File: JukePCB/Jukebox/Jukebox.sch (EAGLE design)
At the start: 31 parts, among them CN1 1X4-BIG

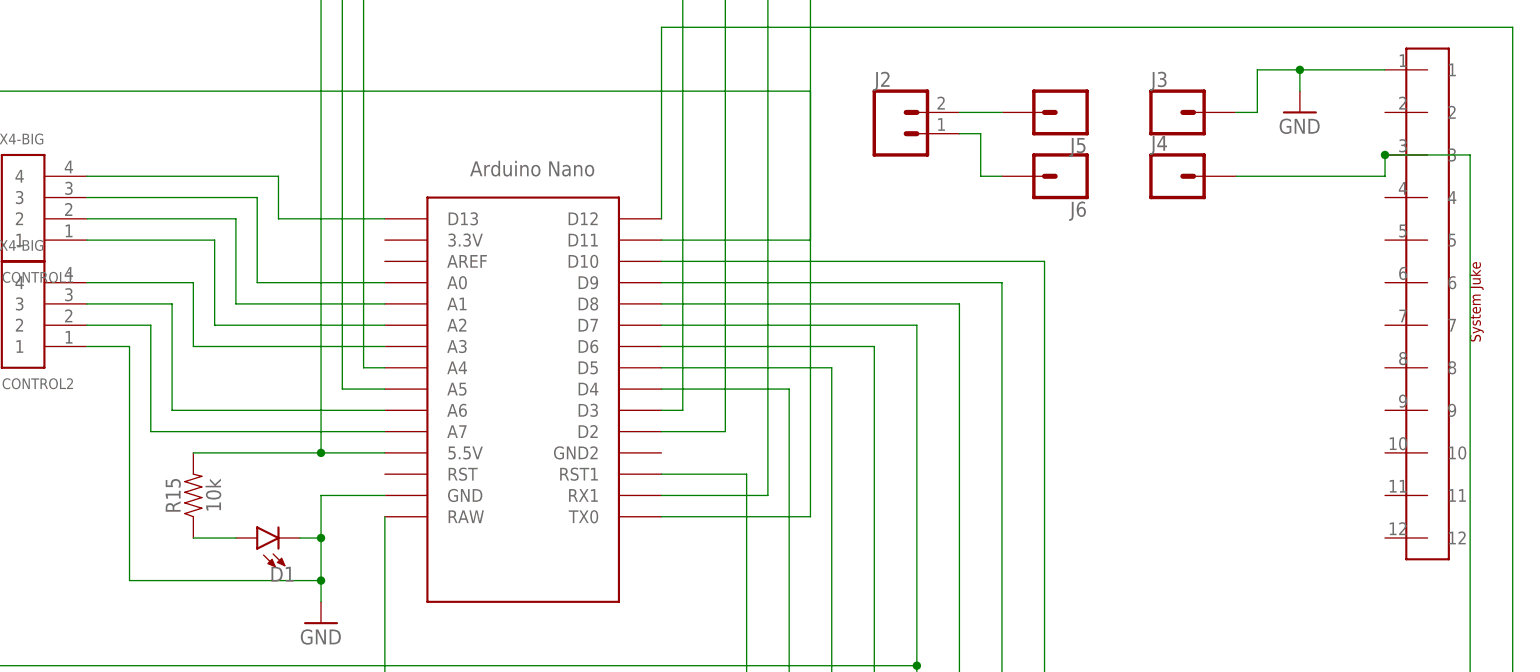
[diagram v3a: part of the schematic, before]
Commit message: board proto 1
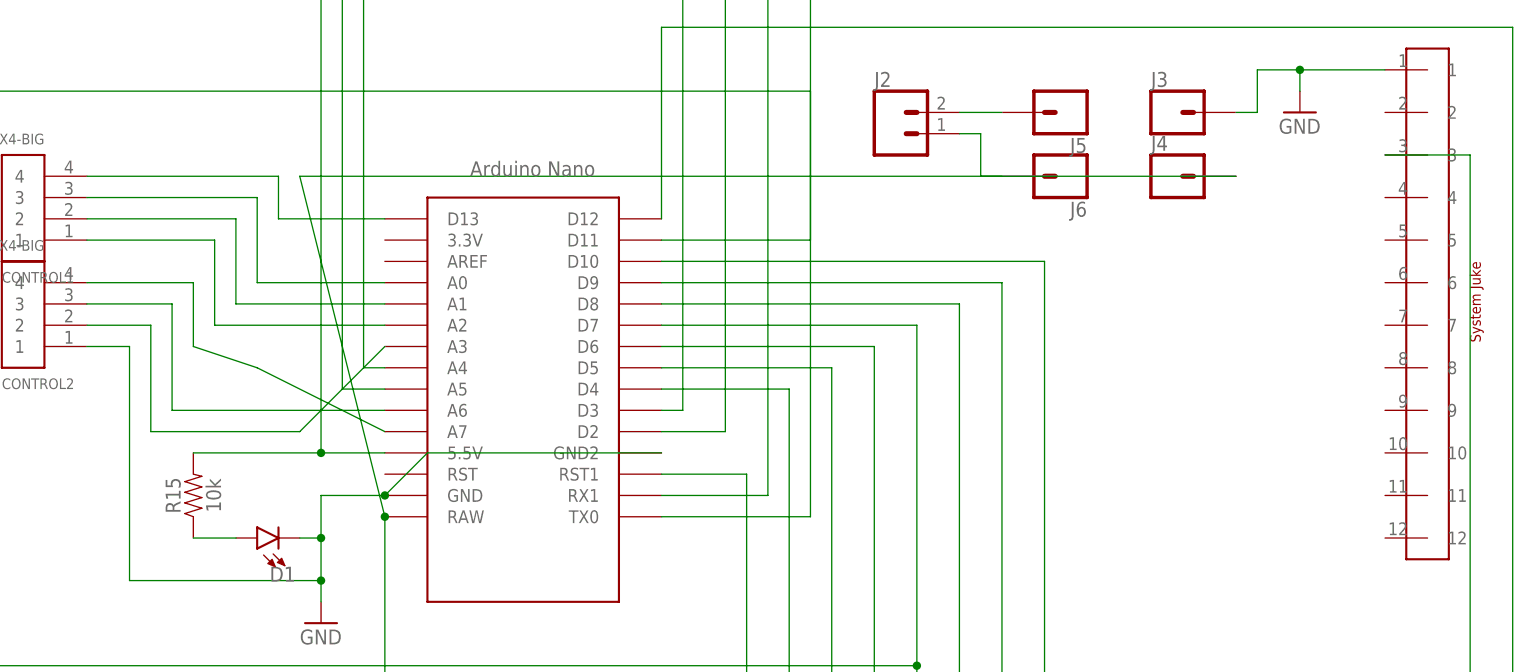
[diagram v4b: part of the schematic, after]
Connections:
- net GND: now also U$1.GND2
- net N$31: now also U$1.A7; no longer U$1.A3
- net N$32: now also J4.1
- net N$36: now also U$1.A3; no longer U$1.A7
- net N$8: no longer J4.1
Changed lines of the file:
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@@
 <wire x1="86.36" y1="-55.88" x2="86.36" y2="2.54" width="0.1524" layer="91"/>
 <pinref part="U$1" gate="G$1" pin="D10"/>
-<wire x1="86.36" y1="2.54" x2="40.64" y2="2.54" width="0.1524" layer="91"/>
+<wire x1="40.64" y1="2.54" x2="86.36" y2="2.54" width="0.1524" layer="91"/>
 </segment>
 </net>
@@
 <pinref part="U$14" gate="G$1" pin="3"/>
 <wire x1="137.16" y1="-127" x2="68.58" y2="-127" width="0.1524" layer="91"/>
-<pinref part="J4" gate="G$1" pin="1"/>
-<wire x1="109.22" y1="12.7" x2="127" y2="12.7" width="0.1524" layer="91"/>
-<wire x1="127" y1="12.7" x2="127" y2="15.24" width="0.1524" layer="91"/>
-<junction x="127" y="15.24"/>
 </segment>
 </net>
@@
 <wire x1="45.72" y1="-93.98" x2="7.62" y2="-93.98" width="0.1524" layer="91"/>
 <wire x1="7.62" y1="-93.98" x2="7.62" y2="-27.94" width="0.1524" layer="91"/>
+<pinref part="J4" gate="G$1" pin="1"/>
+<wire x1="109.22" y1="12.7" x2="-2.54" y2="12.7" width="0.1524" layer="91"/>
+<wire x1="-2.54" y1="12.7" x2="7.62" y2="-27.94" width="0.1524" layer="91"/>
+<junction x="7.62" y="-27.94"/>
 </segment>
 </net>
@@
 <pinref part="CONTROL2" gate="G$1" pin="1"/>
 <wire x1="-22.86" y1="-7.62" x2="-27.94" y2="-7.62" width="0.1524" layer="91"/>
+<pinref part="U$1" gate="G$1" pin="GND2"/>
+<wire x1="40.64" y1="-20.32" x2="12.7" y2="-20.32" width="0.1524" layer="91"/>
+<wire x1="12.7" y1="-20.32" x2="7.62" y2="-25.4" width="0.1524" layer="91"/>
+<junction x="7.62" y="-25.4"/>
 </segment>
 </net>
@@
 <wire x1="-27.94" y1="0" x2="-15.24" y2="0" width="0.1524" layer="91"/>
 <wire x1="-15.24" y1="0" x2="-15.24" y2="-7.62" width="0.1524" layer="91"/>
-<pinref part="U$1" gate="G$1" pin="A3"/>
-<wire x1="-15.24" y1="-7.62" x2="7.62" y2="-7.62" width="0.1524" layer="91"/>
+<pinref part="U$1" gate="G$1" pin="A7"/>
+<wire x1="-15.24" y1="-7.62" x2="-7.62" y2="-10.16" width="0.1524" layer="91"/>
+<wire x1="-7.62" y1="-10.16" x2="7.62" y2="-17.78" width="0.1524" layer="91"/>
 </segment>
 </net>
@@
 <wire x1="-27.94" y1="-5.08" x2="-20.32" y2="-5.08" width="0.1524" layer="91"/>
 <wire x1="-20.32" y1="-5.08" x2="-20.32" y2="-17.78" width="0.1524" layer="91"/>
-<pinref part="U$1" gate="G$1" pin="A7"/>
-<wire x1="-20.32" y1="-17.78" x2="7.62" y2="-17.78" width="0.1524" layer="91"/>
-</segment>
-</net>
+<pinref part="U$1" gate="G$1" pin="A3"/>
+<wire x1="-20.32" y1="-17.78" x2="-2.54" y2="-17.78" width="0.1524" layer="91"/>
+<wire x1="-2.54" y1="-17.78" x2="7.62" y2="-7.62" width="0.1524" layer="91"/>
+</segment>
+</net>

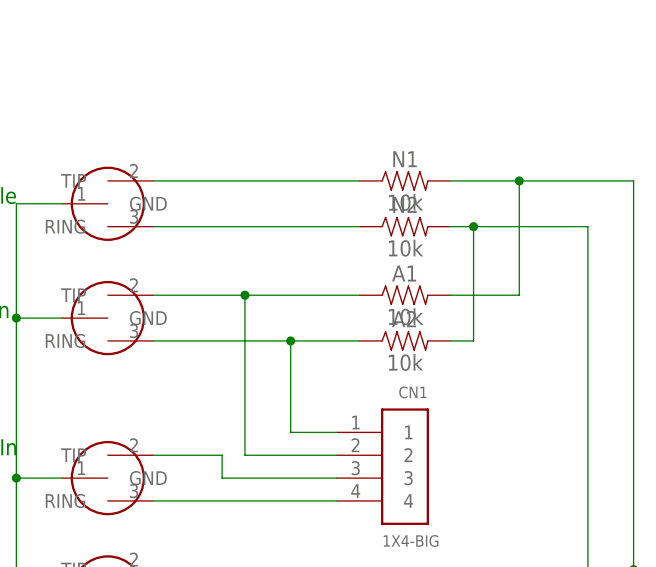
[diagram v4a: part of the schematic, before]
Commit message: almost final routes
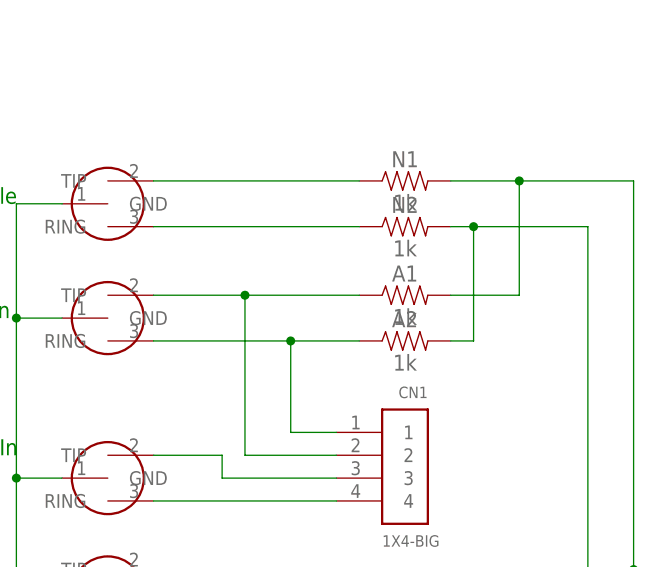
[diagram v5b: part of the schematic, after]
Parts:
- A1, A2, N1, N2: value 10k -> 1k
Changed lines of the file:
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@@
 <part name="TOAMP" library="Jukebox" deviceset="JUKEHEADPHONE" device=""/>
 <part name="AUXOUT" library="Jukebox" deviceset="JUKEHEADPHONE" device=""/>
-<part name="N1" library="SparkFun-Resistors" deviceset="10KOHM" device="-HORIZ-1/4W-1%" value="10k"/>
-<part name="N2" library="SparkFun-Resistors" deviceset="10KOHM" device="-HORIZ-1/4W-1%" value="10k"/>
-<part name="A1" library="SparkFun-Resistors" deviceset="10KOHM" device="-HORIZ-1/4W-1%" value="10k"/>
-<part name="A2" library="SparkFun-Resistors" deviceset="10KOHM" device="-HORIZ-1/4W-1%" value="10k"/>
+<part name="N1" library="SparkFun-Resistors" deviceset="10KOHM" device="-HORIZ-1/4W-1%" value="1k"/>
+<part name="N2" library="SparkFun-Resistors" deviceset="10KOHM" device="-HORIZ-1/4W-1%" value="1k"/>
+<part name="A1" library="SparkFun-Resistors" deviceset="10KOHM" device="-HORIZ-1/4W-1%" value="1k"/>
+<part name="A2" library="SparkFun-Resistors" deviceset="10KOHM" device="-HORIZ-1/4W-1%" value="1k"/>
 <part name="TOLIGHT" library="Jukebox" deviceset="JUKEHEADPHONE" device=""/>
 <part name="R15" library="SparkFun-Resistors" deviceset="10KOHM" device="-HORIZ-1/4W-1%" value="10k"/>

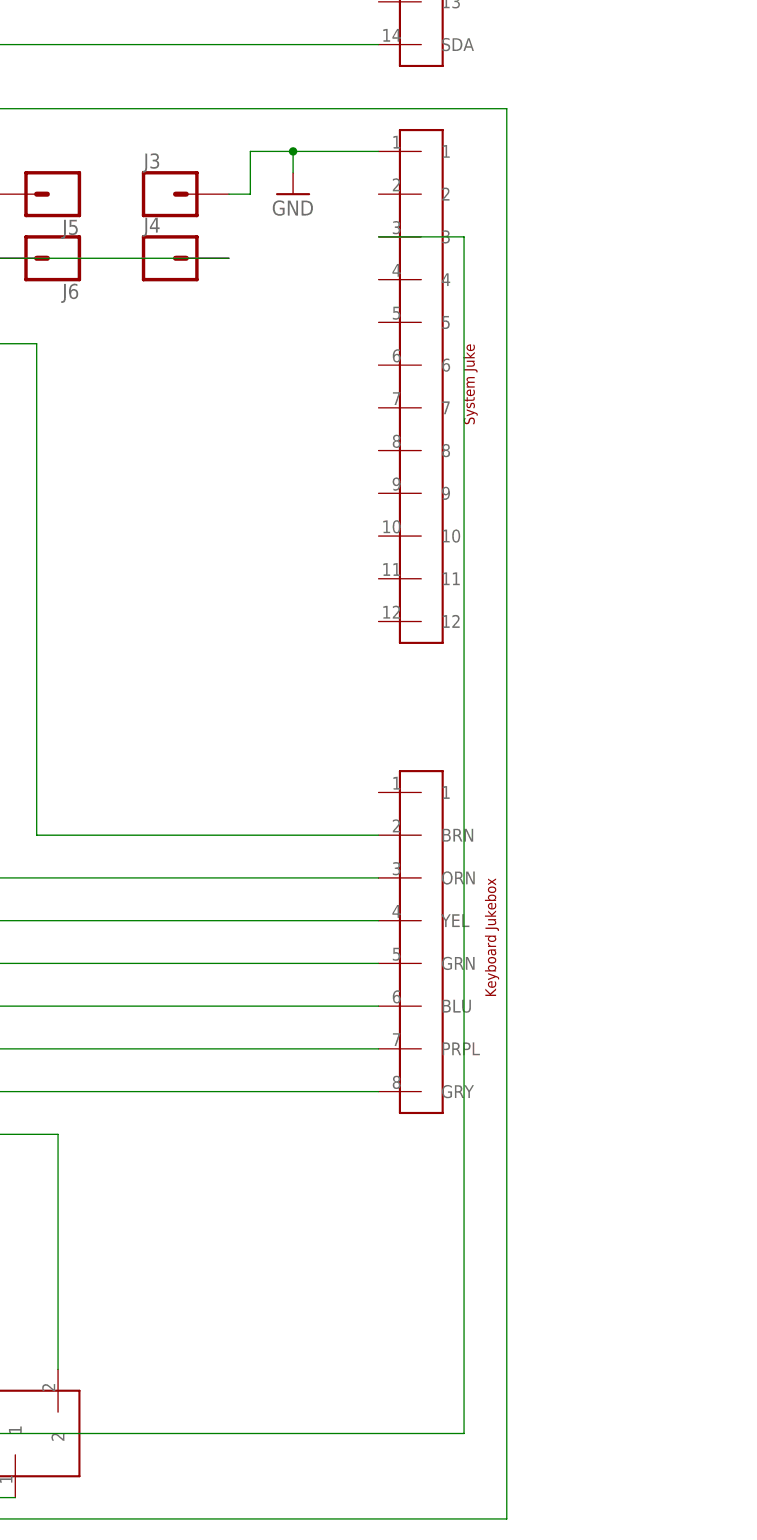
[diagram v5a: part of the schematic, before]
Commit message: Anime.mp4
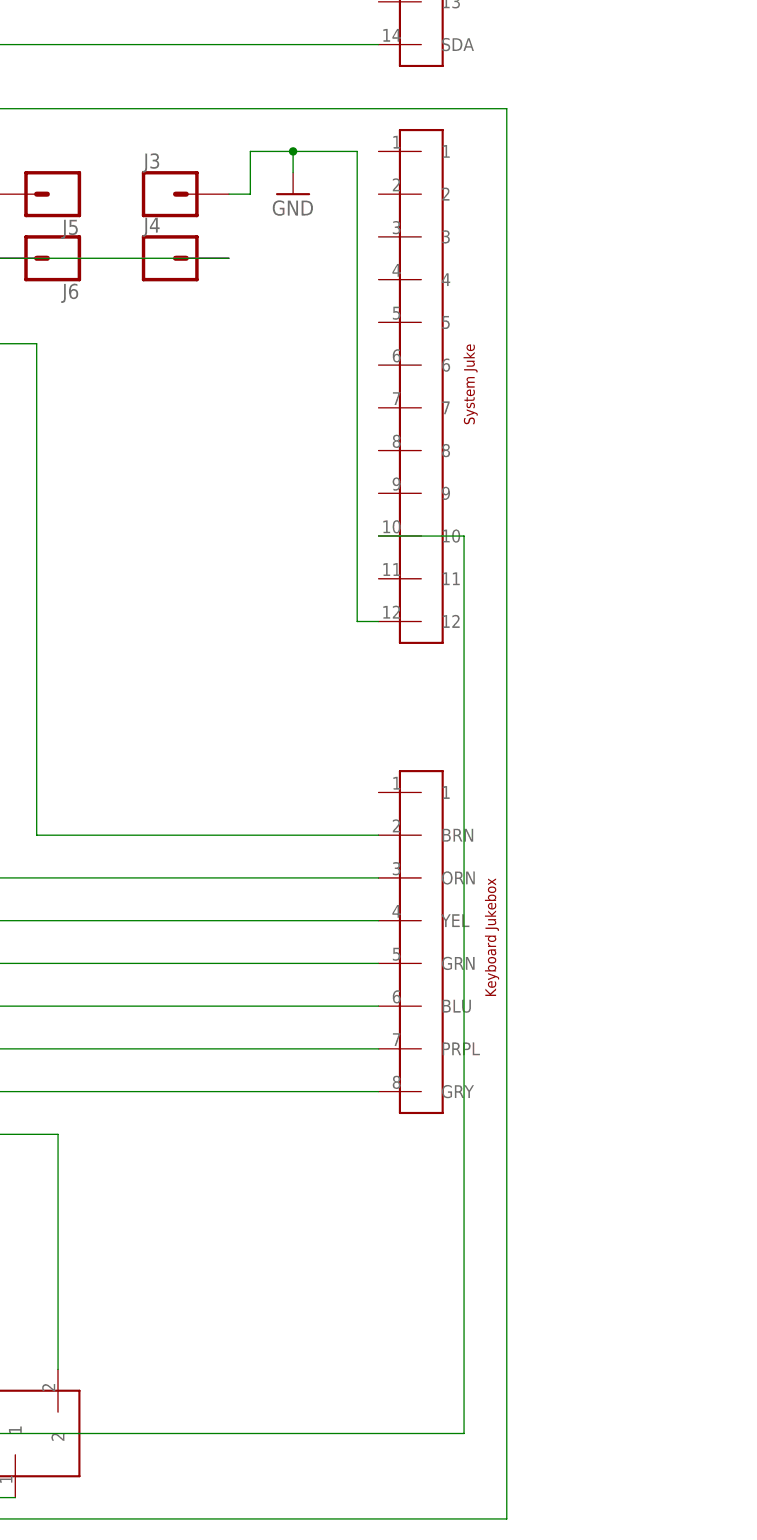
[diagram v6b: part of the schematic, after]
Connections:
- net GND: now also U$8.12; no longer U$8.1
- net N$8: now also U$8.10; no longer U$8.3
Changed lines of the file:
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@@
 <net name="N$8" class="0">
 <segment>
-<pinref part="U$8" gate="G$1" pin="3"/>
-<wire x1="127" y1="15.24" x2="137.16" y2="15.24" width="0.1524" layer="91"/>
-<wire x1="137.16" y1="15.24" x2="137.16" y2="-127" width="0.1524" layer="91"/>
 <pinref part="U$14" gate="G$1" pin="3"/>
 <wire x1="137.16" y1="-127" x2="68.58" y2="-127" width="0.1524" layer="91"/>
+<wire x1="137.16" y1="-127" x2="137.16" y2="-20.32" width="0.1524" layer="91"/>
+<pinref part="U$8" gate="G$1" pin="10"/>
+<wire x1="137.16" y1="-20.32" x2="127" y2="-20.32" width="0.1524" layer="91"/>
 </segment>
 </net>
@@
 </segment>
 <segment>
-<pinref part="U$8" gate="G$1" pin="1"/>
 <pinref part="GND3" gate="1" pin="GND"/>
-<wire x1="127" y1="25.4" x2="116.84" y2="25.4" width="0.1524" layer="91"/>
 <wire x1="116.84" y1="25.4" x2="116.84" y2="22.86" width="0.1524" layer="91"/>
 <pinref part="J3" gate="G$1" pin="1"/>
@@
 <wire x1="111.76" y1="20.32" x2="111.76" y2="25.4" width="0.1524" layer="91"/>
 <wire x1="111.76" y1="25.4" x2="116.84" y2="25.4" width="0.1524" layer="91"/>
+<wire x1="116.84" y1="25.4" x2="124.46" y2="25.4" width="0.1524" layer="91"/>
+<wire x1="124.46" y1="25.4" x2="124.46" y2="-30.48" width="0.1524" layer="91"/>
 <junction x="116.84" y="25.4"/>
+<pinref part="U$8" gate="G$1" pin="12"/>
+<wire x1="124.46" y1="-30.48" x2="127" y2="-30.48" width="0.1524" layer="91"/>
 </segment>
 <segment>
